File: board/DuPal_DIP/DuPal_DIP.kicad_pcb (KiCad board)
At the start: 2 copper layers, 41 parts, among them J1 AVR-ISP-6, J2 RS232, J3 Power IN, SW1 SW_Push, SW2 Power, U1 ATmega8A-PU, U2 74HC595, U3 74HC595, U5 PAL16L8, U6 MAX232, U7 L7805, Y1 8Mhz

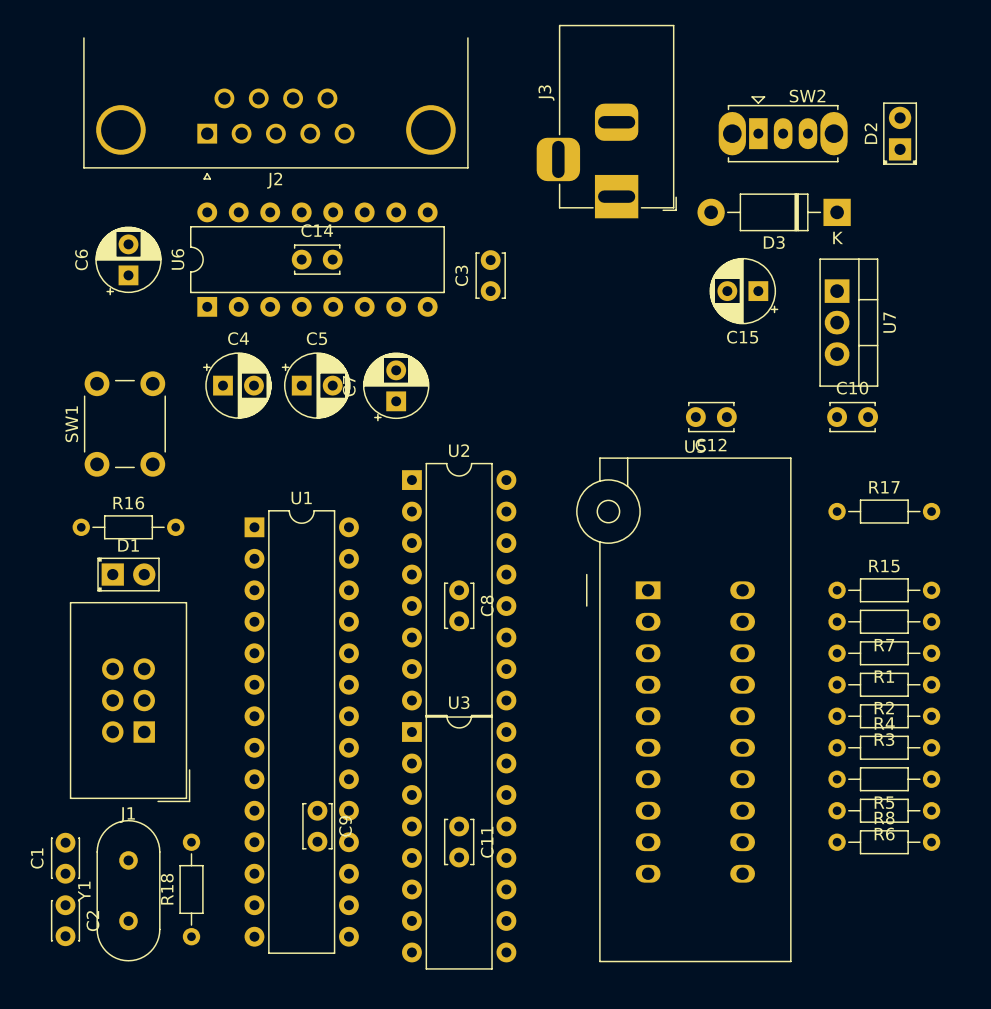
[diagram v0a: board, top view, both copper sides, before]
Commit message: DuPAL project
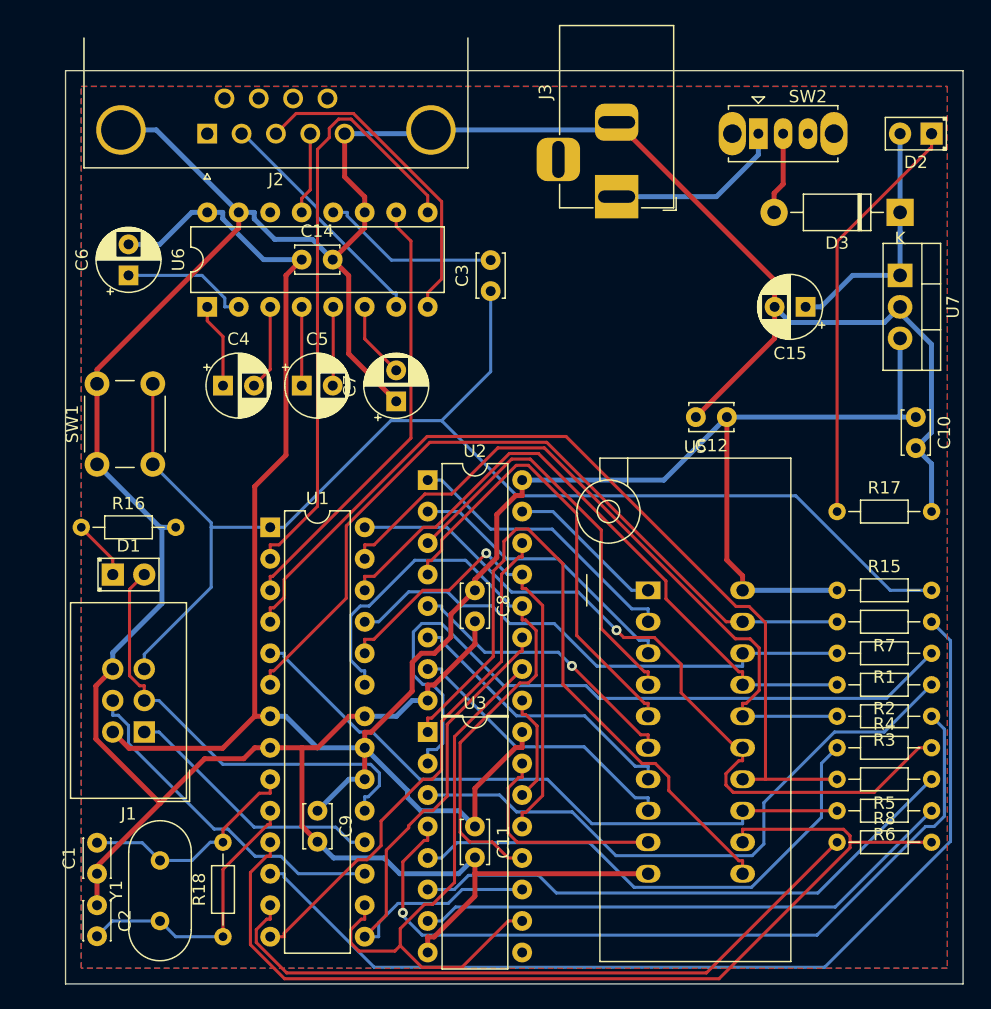
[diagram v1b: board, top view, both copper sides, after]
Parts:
- moved C10 6.35 mm to (95.2, 97.8), turned to 270 degrees
- moved U7 5.24 mm to (94.0, 86.4)
- moved D3 5.08 mm to (94.0, 81.3)
- moved C15 4.02 mm to (86.4, 88.9)
- moved D2 2.84 mm to (96.5, 74.9), turned to 180 degrees
- moved C1 2.54 mm to (29.2, 134.6)
- moved C2 2.54 mm to (29.2, 137.2)
- moved R18 2.54 mm to (39.4, 139.7)
- moved Y1 2.54 mm to (34.3, 138.4)
- moved U1 1.27 mm to (43.2, 106.7)
- moved U2 1.27 mm to (55.9, 102.9)
- moved U3 1.27 mm to (55.9, 123.2)
- moved C11 1.27 mm to (59.7, 130.8)
- moved C8 1.27 mm to (59.7, 111.8)
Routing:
- net GND: track 0.00 -> 280.5 mm
- net VCC: track 0.00 -> 197.5 mm
- net /~RESET: track 0.00 -> 106.6 mm
- net Net-(R7-Pad1): track 0.00 -> 80.7 mm
- net /PAL_TRIO2: track 0.00 -> 80.4 mm
- net /PAL_IO5: track 0.00 -> 74.1 mm
- net Net-(R3-Pad1): track 0.00 -> 65.0 mm, vias 0 -> 1
- net /PAL_TRIO1: track 0.00 -> 63.9 mm
- net /PAL_IO4: track 0.00 -> 61.5 mm, vias 0 -> 1
- net Net-(R1-Pad1): track 0.00 -> 59.0 mm
- net /PAL_IO3: track 0.00 -> 56.7 mm
- net /PAL_I10: track 0.00 -> 56.2 mm
- net Net-(R8-Pad1): track 0.00 -> 55.9 mm
- net /PAL_IO6: track 0.00 -> 52.6 mm
- net /PAL_IO2: track 0.00 -> 52.5 mm
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- added copper zone on B.Cu, net GND
- added copper zone on F.Cu, net GND
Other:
- board outline added: 72.4 x 73.7 mm
